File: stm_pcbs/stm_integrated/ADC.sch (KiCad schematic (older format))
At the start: 10 parts, among them P5 BNC, U16 LT1019ACS8, U17 LTC1859

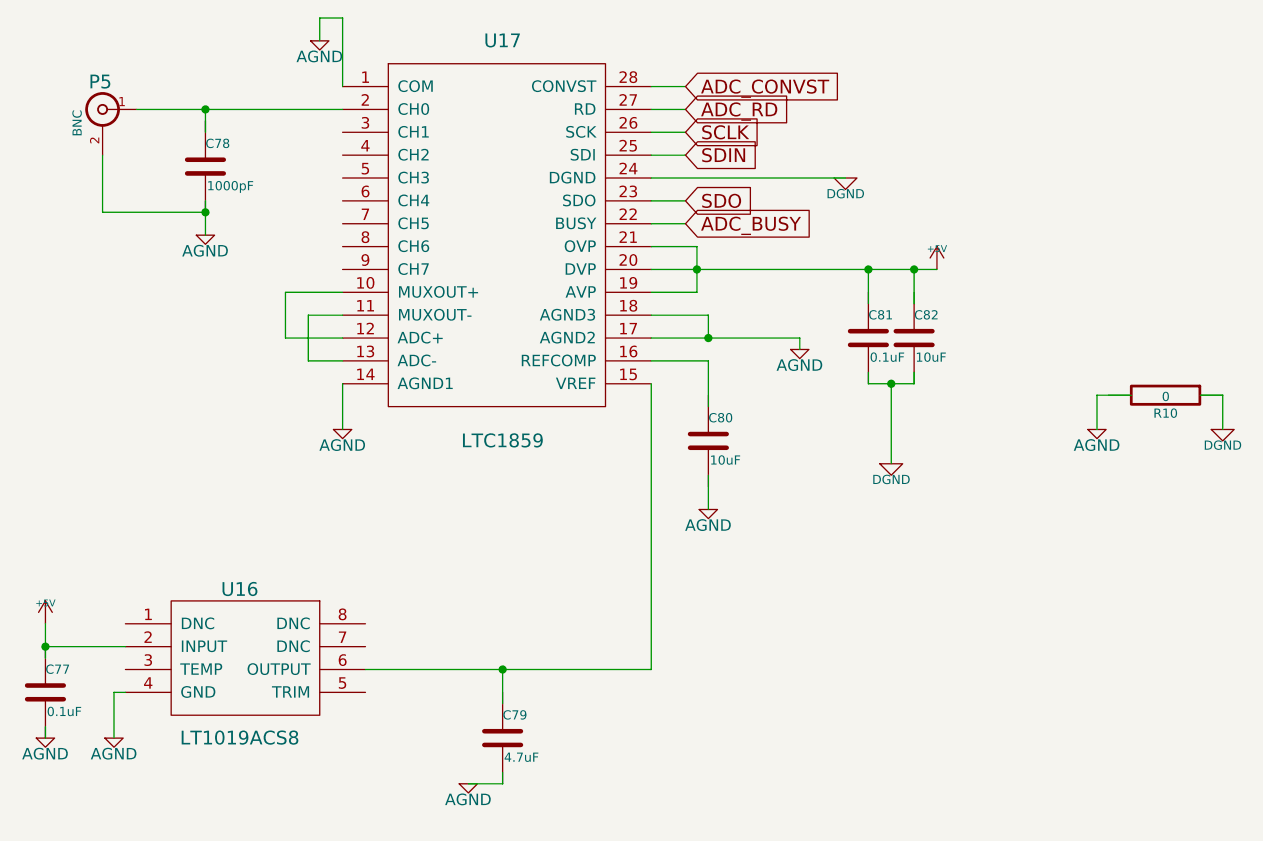
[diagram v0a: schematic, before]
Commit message: fixing more borkage
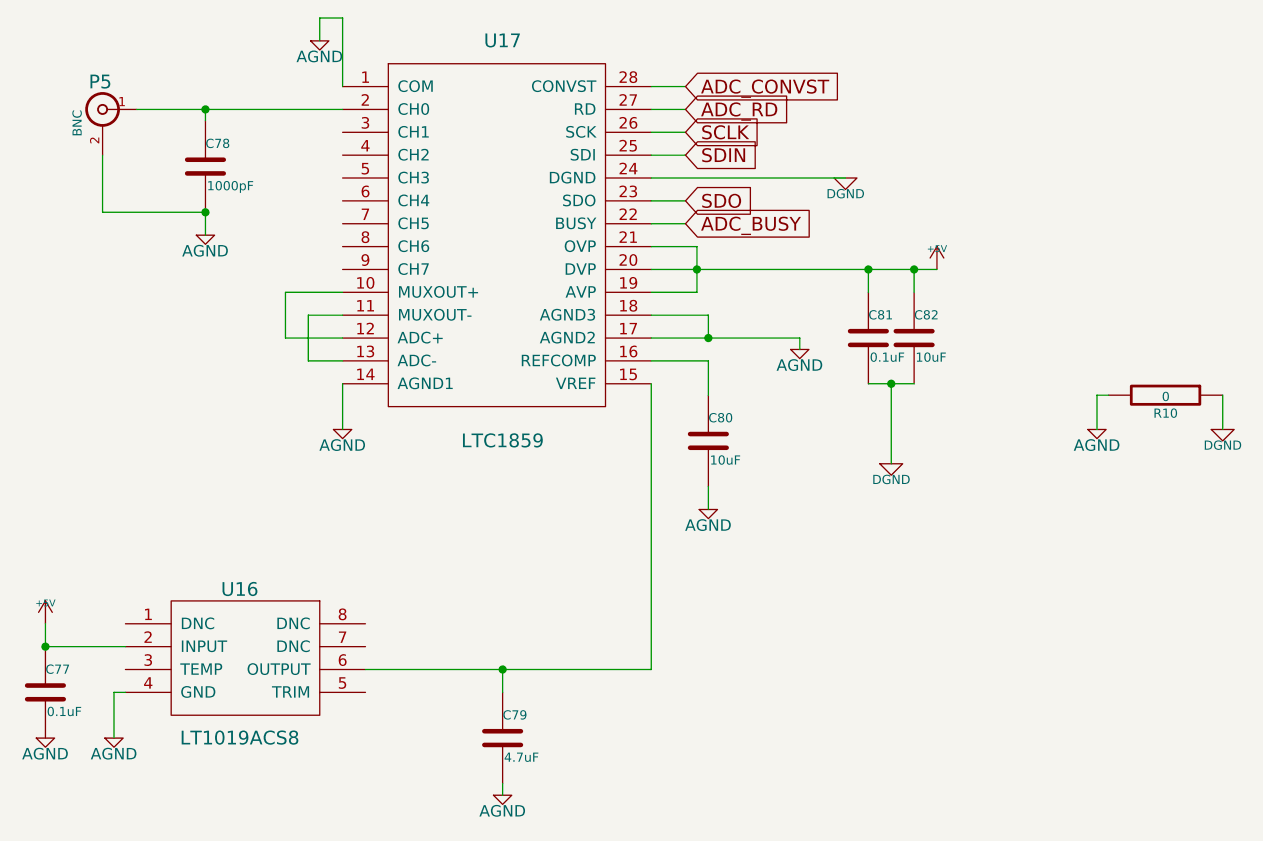
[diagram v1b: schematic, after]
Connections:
- wire segments 63 -> 56
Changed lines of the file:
@@
 L power:AGND #PWR068
 U 1 1 5A233E6E
-P 5100 6000
-F 0 "#PWR068" H 5100 6000 40  0001 C CNN
-F 1 "AGND" H 5100 5930 50  0000 C CNN
-F 2 "" H 5100 6000 60  0000 C CNN
-F 3 "" H 5100 6000 60  0000 C CNN
-	1    5100 6000
+P 5250 6050
+F 0 "#PWR068" H 5250 6050 40  0001 C CNN
+F 1 "AGND" H 5250 5980 50  0000 C CNN
+F 2 "" H 5250 6050 60  0000 C CNN
+F 3 "" H 5250 6050 60  0000 C CNN
+	1    5250 6050
 	1    0    0    -1
 $EndComp
@@
 Connection ~ 6150 4050
 Wire Wire Line
-	6150 4650 6150 4800
-Wire Wire Line
-	6150 4150 6150 4350
-Wire Wire Line
 	6150 4150 5900 4150
-Wire Wire Line
-	3650 3050 3950 3050
-Wire Wire Line
-	3950 3050 3950 3150
 Wire Wire Line
 	4550 4250 4550 4450
@@
 Connection ~ 6950 4250
 Wire Wire Line
-	4650 5500 5250 5500
-Wire Wire Line
 	5900 5500 5900 4250
 Wire Wire Line
 	3600 5400 3250 5400
 Wire Wire Line
-	5100 6000 5250 6000
+	5250 6050 5250 6000
 Wire Wire Line
 	3600 5600 3550 5600
@@
 Wire Wire Line
 	3250 5300 3250 5400
-Connection ~ 3950 3050
-Wire Wire Line
-	5250 5500 5250 5650
-Connection ~ 5250 5500
 Wire Wire Line
 	8400 4300 8400 4450
 Wire Wire Line
-	7850 4300 8000 4300
+	7850 4300 7900 4300
 Wire Wire Line
 	7850 4300 7850 4450
 Wire Wire Line
-	7050 3750 7050 3900
-Connection ~ 7050 3750
-Wire Wire Line
-	6850 3750 6850 3900
+	6850 3750 6850 3850
 Connection ~ 6850 3750
-Wire Wire Line
-	5250 6000 5250 5950
 Connection ~ 3250 5400
-Wire Wire Line
-	3250 5750 3250 5800
-Wire Wire Line
-	6850 4200 6850 4250
-Wire Wire Line
-	7050 4250 7050 4200
-Wire Wire Line
-	8400 4300 8300 4300
-Wire Wire Line
-	3950 3450 3950 3500
 Wire Wire Line
 	3950 3500 3500 3500
@@
 Wire Wire Line
 	6950 4250 7050 4250
-Wire Wire Line
-	3950 3050 4550 3050
-Wire Wire Line
-	5250 5500 5900 5500
-Wire Wire Line
-	7050 3750 7150 3750
-Wire Wire Line
-	6850 3750 7050 3750
-Wire Wire Line
-	3250 5400 3250 5450
 Wire Wire Line
 	3950 3500 3950 3600
@@
 Wire Wire Line
 	5900 3550 6050 3550
+Wire Wire Line
+	6850 3750 7050 3750
+Wire Wire Line
+	7050 3850 7050 3750
+Connection ~ 7050 3750
+Wire Wire Line
+	7050 3750 7150 3750
+Wire Wire Line
+	4650 5500 5250 5500
+Wire Wire Line
+	5250 5600 5250 5500
+Connection ~ 5250 5500
+Wire Wire Line
+	5250 5500 5900 5500
+Wire Wire Line
+	3650 3050 3950 3050
+Wire Wire Line
+	3950 3100 3950 3050
+Connection ~ 3950 3050
+Wire Wire Line
+	3950 3050 4550 3050
+Wire Wire Line
+	6150 4300 6150 4150
+Wire Wire Line
+	6150 4800 6150 4700
 $EndSCHEMATC
